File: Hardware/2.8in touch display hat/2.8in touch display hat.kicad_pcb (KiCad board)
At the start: 2 copper layers, 50 x 69 mm, 57 parts, among them J1 B2B (JST-SH), J2 LRA (PicoBlade), Q1 NMOS, U1 DRV2605LDGS, U3 VEML7700-TR, U4 ATECC608B

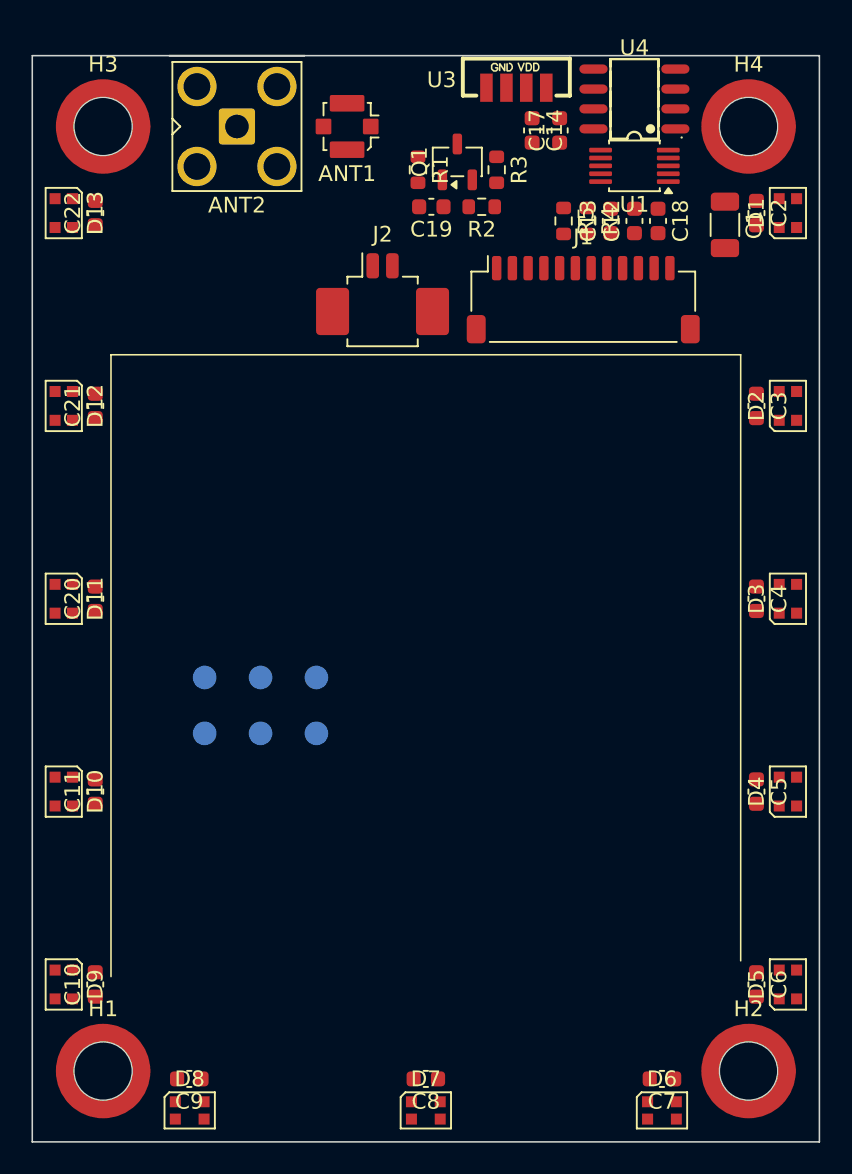
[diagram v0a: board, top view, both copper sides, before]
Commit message: first pass routing
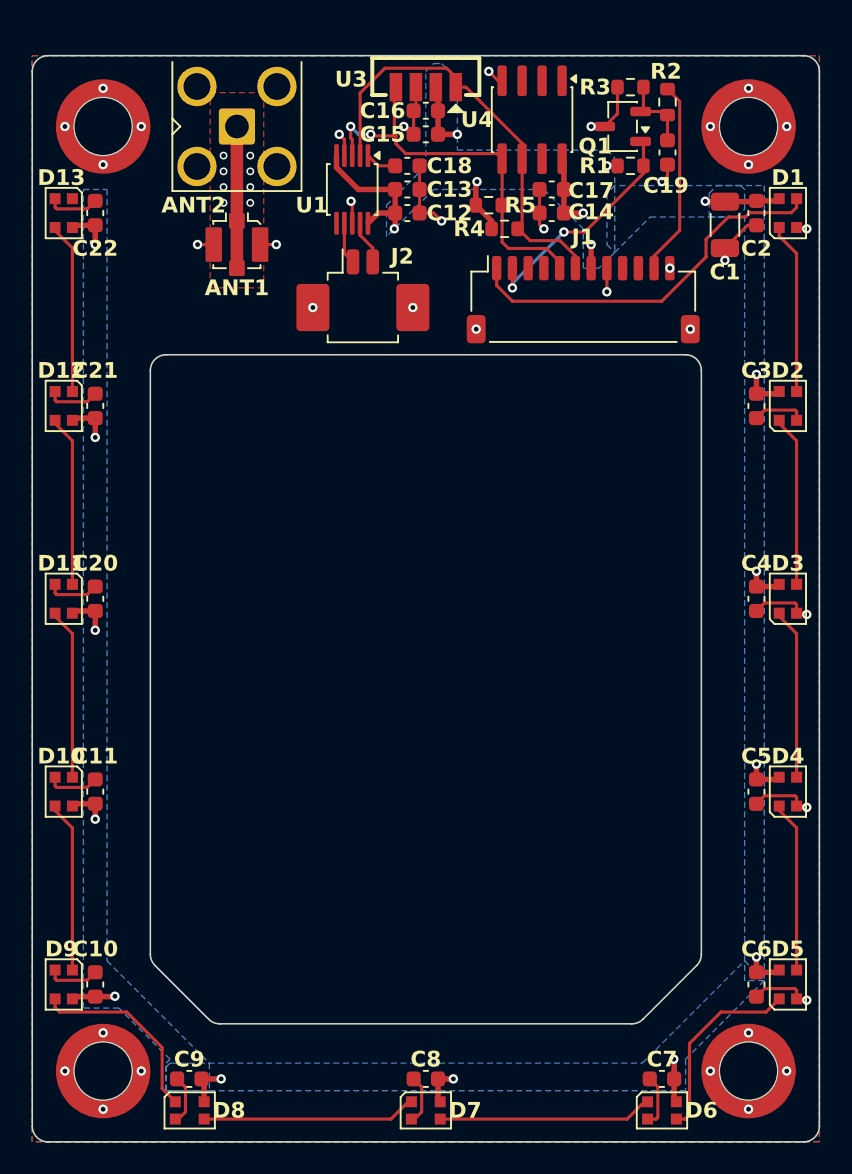
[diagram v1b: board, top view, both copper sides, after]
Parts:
- removed TP1: +3.3V, TestPoint:TestPoint_Pad_D1.5mm
- removed TP2: VBUS, TestPoint:TestPoint_Pad_D1.5mm
- removed TP3: SCL, TestPoint:TestPoint_Pad_D1.5mm
- removed TP4: SDA, TestPoint:TestPoint_Pad_D1.5mm
- removed TP5: LEDS, TestPoint:TestPoint_Pad_D1.5mm
- removed TP6: CHARGE, TestPoint:TestPoint_Pad_D1.5mm
- added C15: 2.2μF, Capacitor_SMD:C_0603_1608Metric, F.Cu at (149.0, 120.0)
- added C16: 100nF, Capacitor_SMD:C_0603_1608Metric, F.Cu at (149.0, 118.5)
- U4: footprint EasyEDA:SOIC-8_L4.9-W3.9-P1.27-LS6.0-BL -> Package_SO:SOIC-8-1EP_3.9x4.9mm_P1.27mm_EP2.29x3mm
- moved G*** 54.8 mm to (117.5, 143.5)
- moved U1 18.0 mm to (144.3, 123.5), turned to -90 degrees
- moved C18 16.3 mm to (147.8, 122.0), turned to 0 degrees
- moved C19 15.4 mm to (164.3, 121.2), turned to -90 degrees
- moved C12 14.4 mm to (147.8, 125.0), turned to 180 degrees
- moved R2 13.5 mm to (164.3, 118.0), turned to -90 degrees
- moved R1 13.5 mm to (162.0, 122.0), turned to 0 degrees
- moved C13 13.1 mm to (147.8, 123.5), turned to 180 degrees
- moved Q1 10.7 mm to (161.5, 119.5), turned to 180 degrees
- moved ANT1 10.3 mm to (137.0, 127.0), turned to 0 degrees
- moved R3 9.99 mm to (162.0, 117.0), turned to 0 degrees
- moved U4 6.63 mm to (155.8, 119.1), turned to -90 degrees
- moved U3 5.75 mm to (149.0, 117.0)
- moved C17 5.27 mm to (157.0, 125.0), turned to 0 degrees
- moved R4 5.27 mm to (154.0, 126.0), turned to 0 degrees
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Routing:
- net GND: track 0.00 -> 69.5 mm, vias 0 -> 45
- net +3.3V: track 0.00 -> 60.7 mm, vias 0 -> 19
- net /SCL: track 0.00 -> 27.7 mm
- net /SDA: track 0.00 -> 25.7 mm, vias 0 -> 2
- net /GPIO15: track 0.00 -> 24.2 mm
- net /CHARGE: track 0.00 -> 14.9 mm, vias 0 -> 2
- net Net-(D7-DOUT): track 0.00 -> 13.6 mm
- net Net-(D6-DOUT): track 0.00 -> 13.6 mm
- net VBUS: track 0.00 -> 12.4 mm
- net Net-(D5-DOUT): track 0.00 -> 12.3 mm
- net Net-(D8-DOUT): track 0.00 -> 12.2 mm
- net Net-(D3-DOUT): track 0.00 -> 10.9 mm
- net Net-(D2-DOUT): track 0.00 -> 10.9 mm
- net Net-(D4-DOUT): track 0.00 -> 10.9 mm
- net Net-(D1-DOUT): track 0.00 -> 10.9 mm
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- added copper zone on B.Cu, net +3.3V
- added copper zone on B.Cu, net GND
- added copper zone on F.Cu, net GND
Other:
- outline, holes or cut-outs redrawn
